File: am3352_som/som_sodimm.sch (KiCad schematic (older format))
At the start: 1 part, among them J1 SODIMM-204

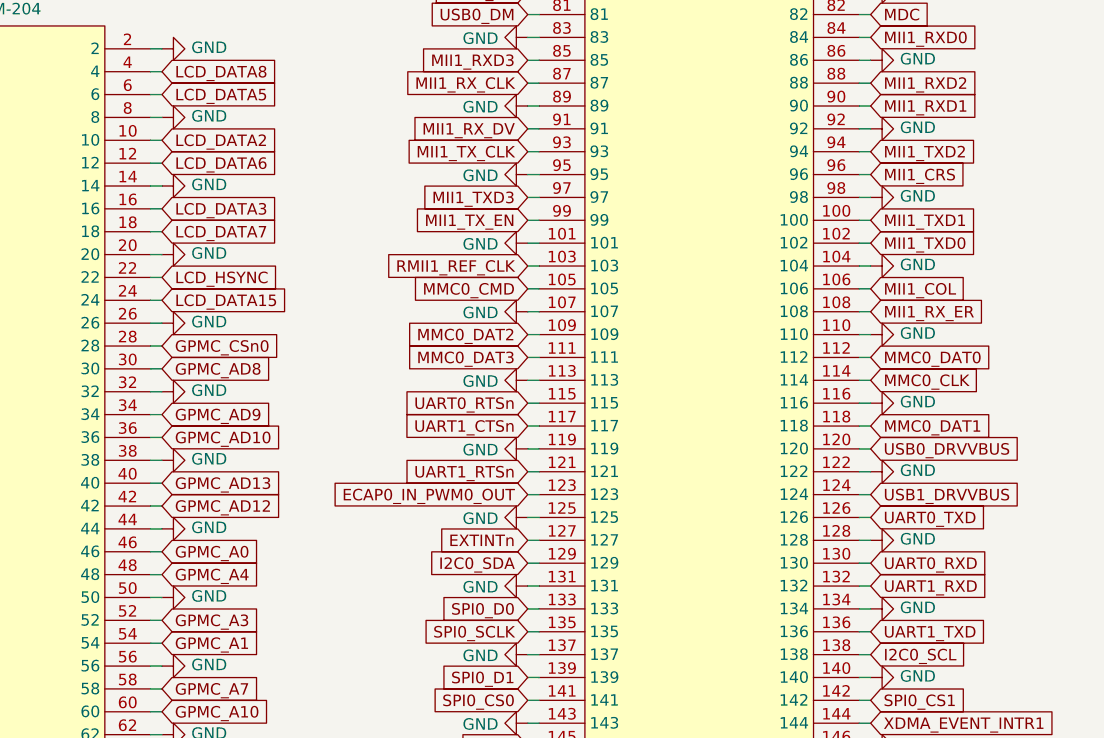
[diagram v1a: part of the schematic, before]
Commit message: adjust
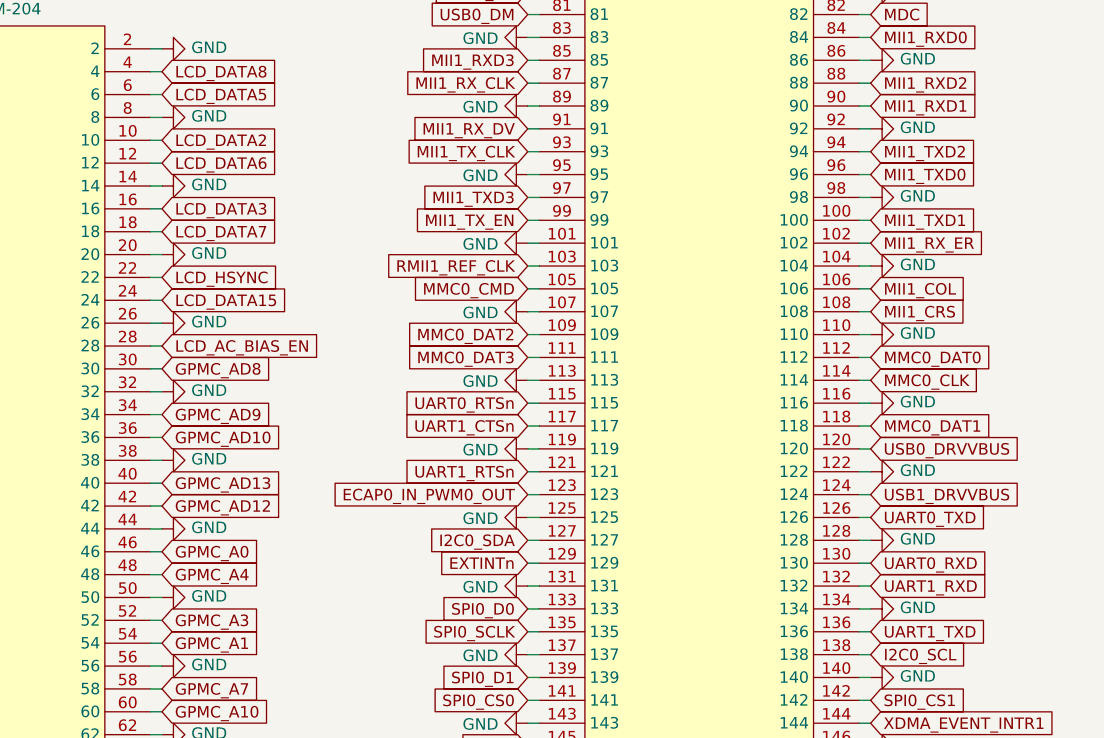
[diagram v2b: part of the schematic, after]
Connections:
- net EXTINTn: now also J1.129; no longer J1.127
- net I2C0_SDA: now also J1.127; no longer J1.129
- net MII1_CRS: now also J1.108; no longer J1.96
- net MII1_RX_ER: now also J1.102; no longer J1.108
- net MII1_TXD0: now also J1.96; no longer J1.102
- net GPMC_CSn0 renamed LCD_AC_BIAS_EN
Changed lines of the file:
@@
 Text GLabel 4850 3500 0    50   Input ~ 0
 ECAP0_IN_PWM0_OUT
+Text GLabel 4850 3800 0    50   Input ~ 0
+EXTINTn
 Text GLabel 4850 3700 0    50   Input ~ 0
-EXTINTn
-Text GLabel 4850 3800 0    50   Input ~ 0
 I2C0_SDA
 Text GLabel 4850 4000 0    50   Input ~ 0
@@
 LCD_DATA15
 Text GLabel 3250 2850 2    50   Input ~ 0
-GPMC_CSn0
+LCD_AC_BIAS_EN
 Text GLabel 3250 2950 2    50   Input ~ 0
 GPMC_AD8
@@
 Text GLabel 6350 2000 2    50   Input ~ 0
 MII1_TXD2
-Text GLabel 6350 2100 2    50   Input ~ 0
+Text GLabel 6350 2700 2    50   Input ~ 0
 MII1_CRS
 Text GLabel 6350 2300 2    50   Input ~ 0
 MII1_TXD1
-Text GLabel 6350 2400 2    50   Input ~ 0
+Text GLabel 6350 2100 2    50   Input ~ 0
 MII1_TXD0
 Text GLabel 6350 2600 2    50   Input ~ 0
 MII1_COL
-Text GLabel 6350 2700 2    50   Input ~ 0
+Text GLabel 6350 2400 2    50   Input ~ 0
 MII1_RX_ER
 Text GLabel 6350 2900 2    50   Input ~ 0
